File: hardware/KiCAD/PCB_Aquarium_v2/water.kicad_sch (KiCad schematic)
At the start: 3 parts, among them J6 Conn_01x03, J7 Conn_01x03, J8 Conn_01x03

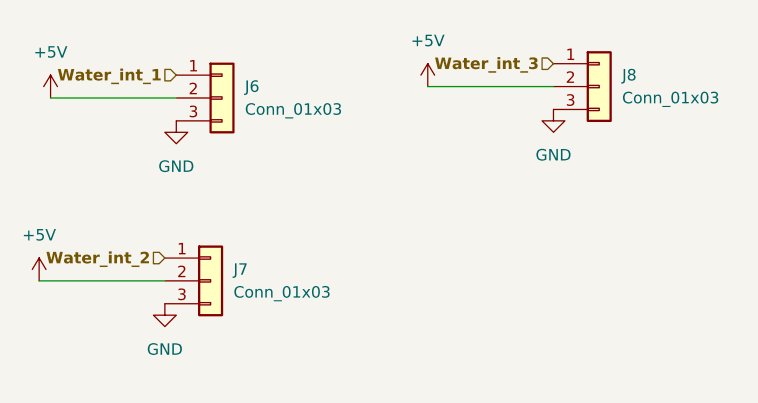
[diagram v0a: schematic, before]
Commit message: PCB principal finis
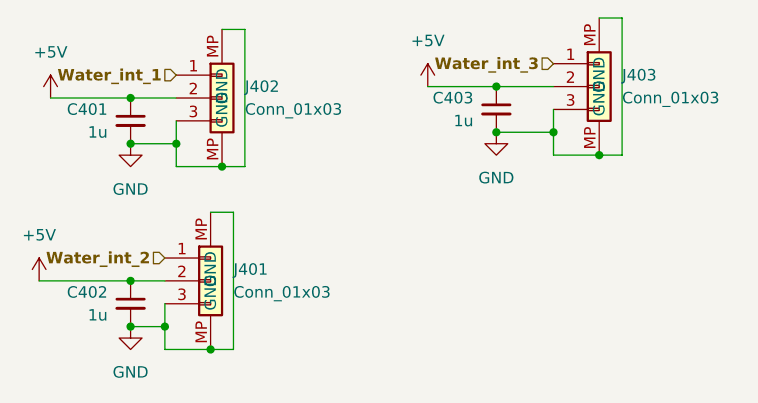
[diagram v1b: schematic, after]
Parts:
- added C401, C402, C403: 1u, Capacitor_SMD:C_0603_1608Metric, symbol Device:C_Small
- J401: renamed from J7; footprint (none) -> Connector_JST:JST_SH_BM03B-SRSS-TB_1x03-1MP_P1.00mm_Vertical; symbol Connector_Generic:Conn_01x03 -> my_lib:JST_SH_3_Vertical
- J402: renamed from J6; footprint (none) -> Connector_JST:JST_SH_BM03B-SRSS-TB_1x03-1MP_P1.00mm_Vertical; symbol Connector_Generic:Conn_01x03 -> my_lib:JST_SH_3_Vertical
- J403: renamed from J8; footprint (none) -> Connector_JST:JST_SH_BM03B-SRSS-TB_1x03-1MP_P1.00mm_Vertical; symbol Connector_Generic:Conn_01x03 -> my_lib:JST_SH_3_Vertical
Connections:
- net +5V: now also C401.1, C402.1, C403.1
- net GND: now also J401.MP (GND), J402.MP (GND), J403.MP (GND), C401.2, C402.2, C403.2
